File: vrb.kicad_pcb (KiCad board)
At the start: 6 copper layers, 82 x 75 mm, 224 parts, among them J1 SM04B-GHS, J10 MiniFit, J11 XT30, J12 Mezzanine, J13 MiniFit, J14 Conn_01x02, J2 SM04B-GHS, J3 MiniFit, J4 MiniFit, J5 Pixhawk 1, J6 Pixhawk 2, J7 SM04B-GHS, J8 DEBUG, J9 SM04B-GHS, Q1 Q_NMOS_GSD, Q2 Q_NMOS_GSD, Q3 MMBT5551L, Q4 FDC5614P, U1 STM32G0B1CBUx, U10 INA180A2, U11 TJA1051TK/3/1J, U12 I3A4W008A033V-001-R, U13 INA180A2, U14 TPS2121, U15 TPS2121, U16 TLV71333PDBVR, U17 TLA2528, U18 TPS2116DRL, U2 TJA1051TK/3/1J, U3 LMR51635, U4 INA180A2, U5 LMR51635, U6 INA180A2, U7 LMR51635, U8 INA180A2, U9 LMR51635, Y1 XRCGB16M000FXN20R0

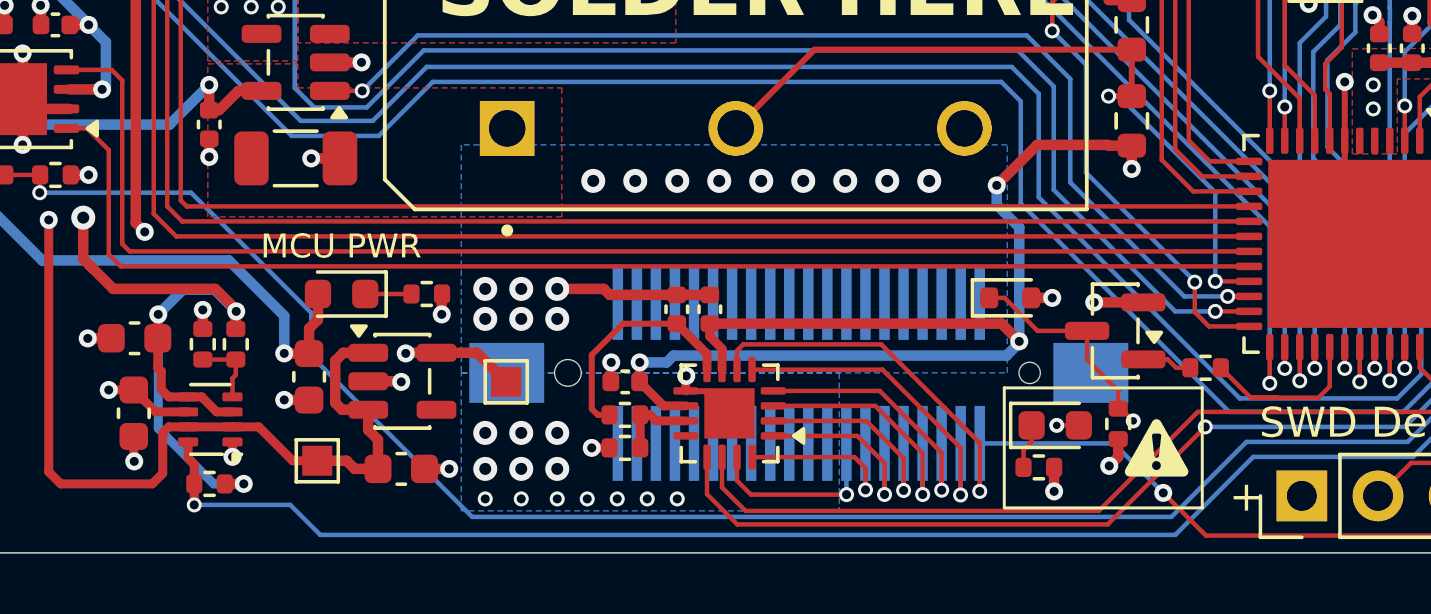
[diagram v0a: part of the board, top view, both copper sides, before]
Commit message: final export of r1 after changes
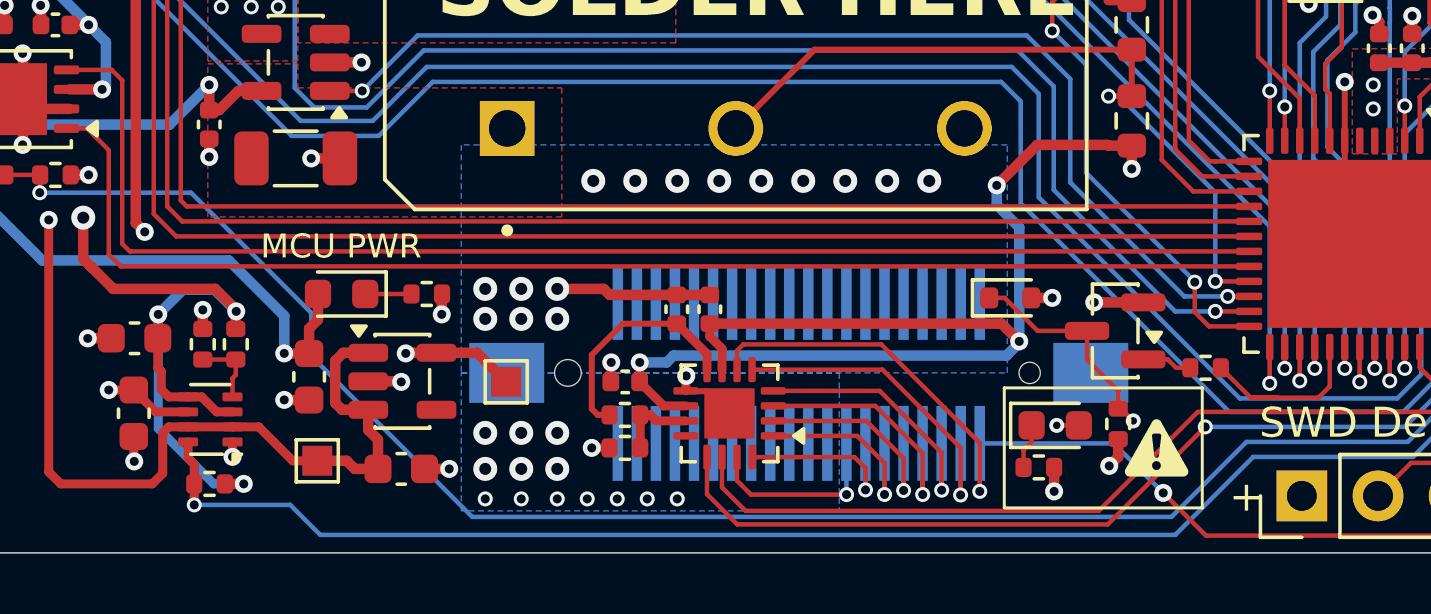
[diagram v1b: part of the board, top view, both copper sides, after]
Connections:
- net /IPAYLOAD renamed /IPAYLOAD1
- net /RESV0 renamed /IPAYLOAD2
- net /RESV1 renamed /IPAYLOAD3
- net /RESV2 renamed /VBAT_SCALED
